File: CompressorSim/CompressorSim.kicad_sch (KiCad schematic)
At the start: 14 parts, among them U1 TL074

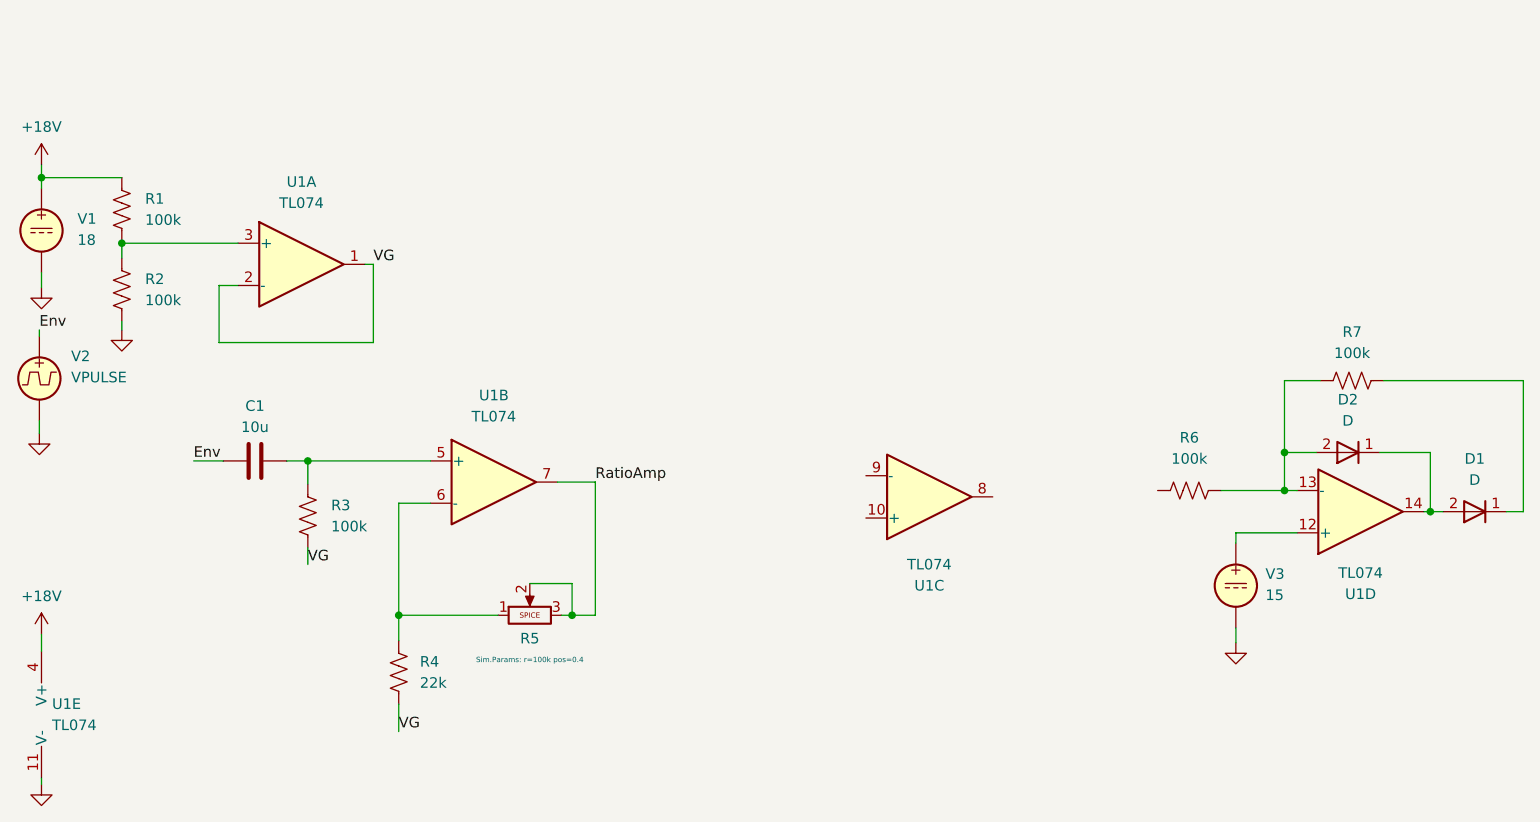
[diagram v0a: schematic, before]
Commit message: compressor simulation
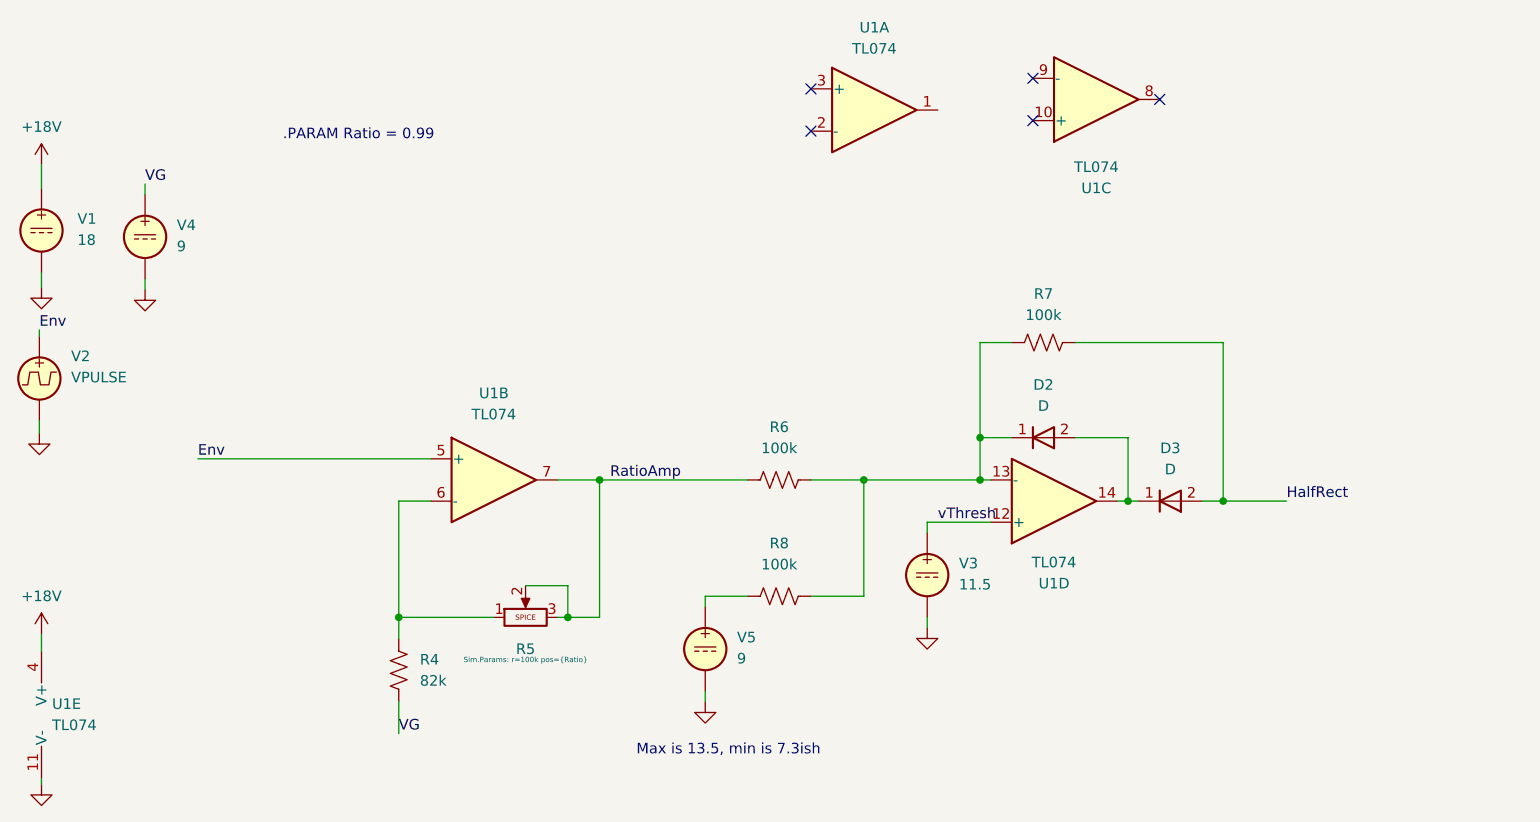
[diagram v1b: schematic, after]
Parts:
- removed C1: 10u, symbol Device:C
- removed D1: D, symbol Simulation_SPICE:D
- removed R1, R2, R3: 100k, symbol Device:R_US
- added D3: D, symbol Simulation_SPICE:D
- added R8: 100k, symbol Device:R_US
- added V4, V5: 9, symbol Simulation_SPICE:VDC
- R4: value 22k -> 82k
- V3: value 15 -> 11.5
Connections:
- net Env: now also U1.5 (+)
- net GND: now also V4.2, V5.2
- net RatioAmp: now also R6.1
- net VG: now also V4.1; no longer U1.1, U1.2 (-)
- net at R6.2, R7.1, U1.13 (-): now also D2.1 (K), R8.2; no longer D2.2 (A)
- net HalfRect: now reaches R7.2
- net HalfRect: now also D3.2 (A)
- net vThresh: now reaches U1.12 (+), V3.1
- net at U1.14: now also D2.2 (A), D3.1 (K); no longer D2.1 (K)
- new net: R8.1, V5.1
- no-connect marks 0 -> 5
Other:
- note added: ".PARAM Ratio = 0.99"
- note added: "Max is 13.5, min is 7.3ish"
- moved on the sheet: D2, R5, R6, R7, U1A, U1C, U1D, V3
